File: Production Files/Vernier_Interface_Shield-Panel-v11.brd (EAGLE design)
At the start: 166.6 x 171.7 mm, 175 parts, among them U1 74HC4052SO, U2 LMV358, U3 74HC4052SO, U4 LMV358, U5 74HC4052SO, U6 LMV358, U7 74HC4052SO, U8 LMV358

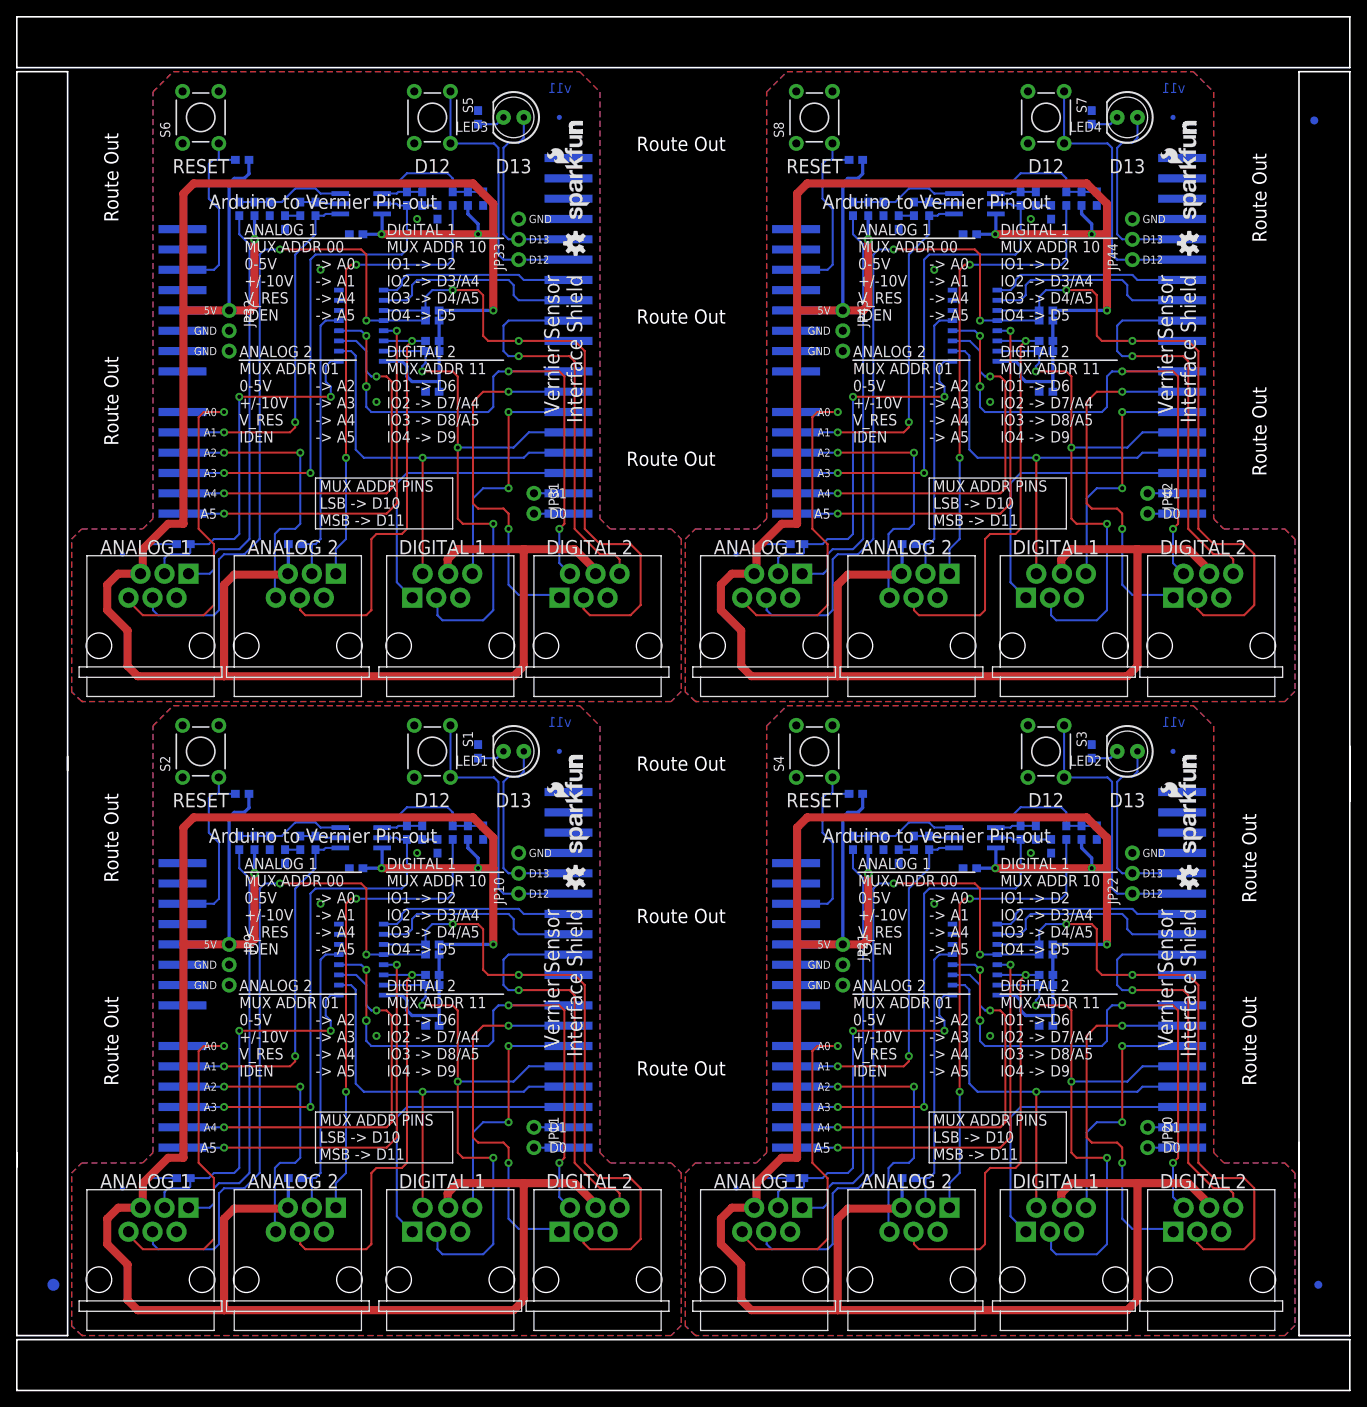
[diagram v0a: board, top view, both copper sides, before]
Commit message: Re-re-created Panel v11
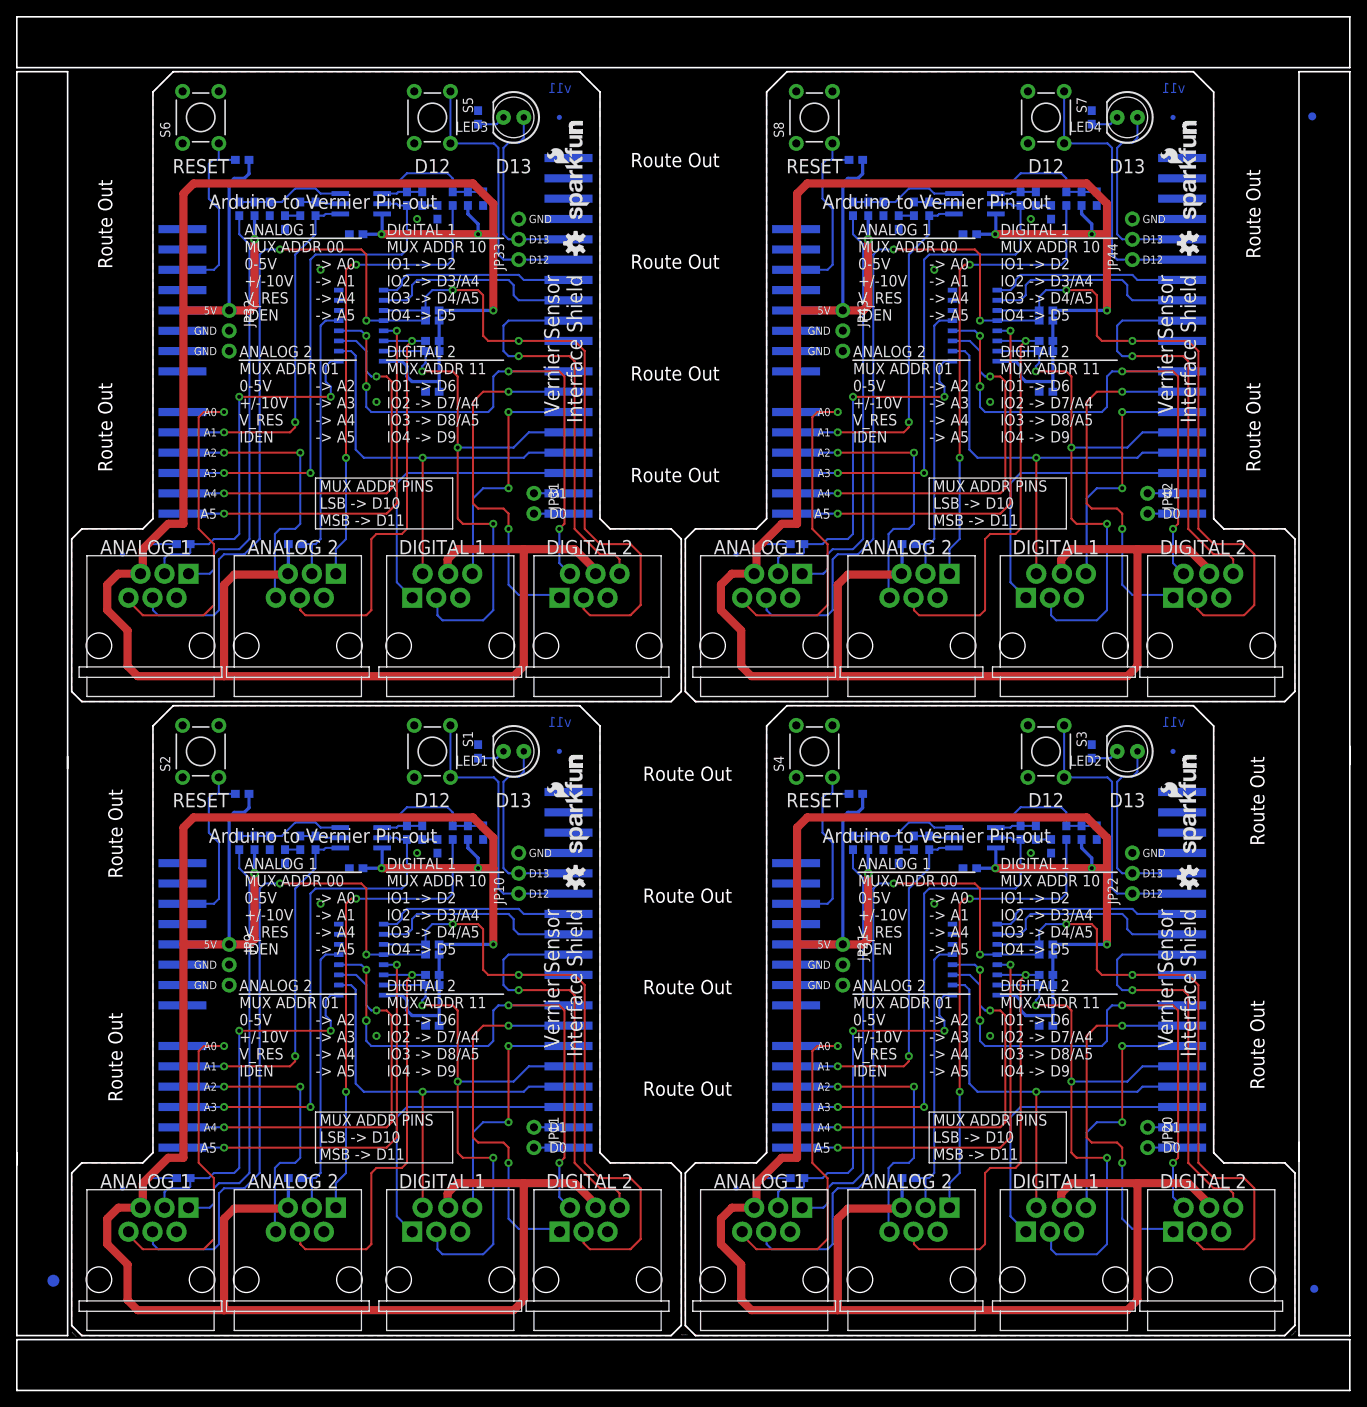
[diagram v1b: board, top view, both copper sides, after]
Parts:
- removed E$5: (no value), SparkFun-Aesthetics:FIDUCIAL-1X2
- added E$6: (no value), SparkFun-Aesthetics:FIDUCIAL-1X2
- moved E$4 0.72 mm to (162.2, 12.7)
- moved E$1 0.51 mm to (4.57, 13.7)
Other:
- outline, holes or cut-outs redrawn
